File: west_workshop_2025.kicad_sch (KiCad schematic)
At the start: 4 parts

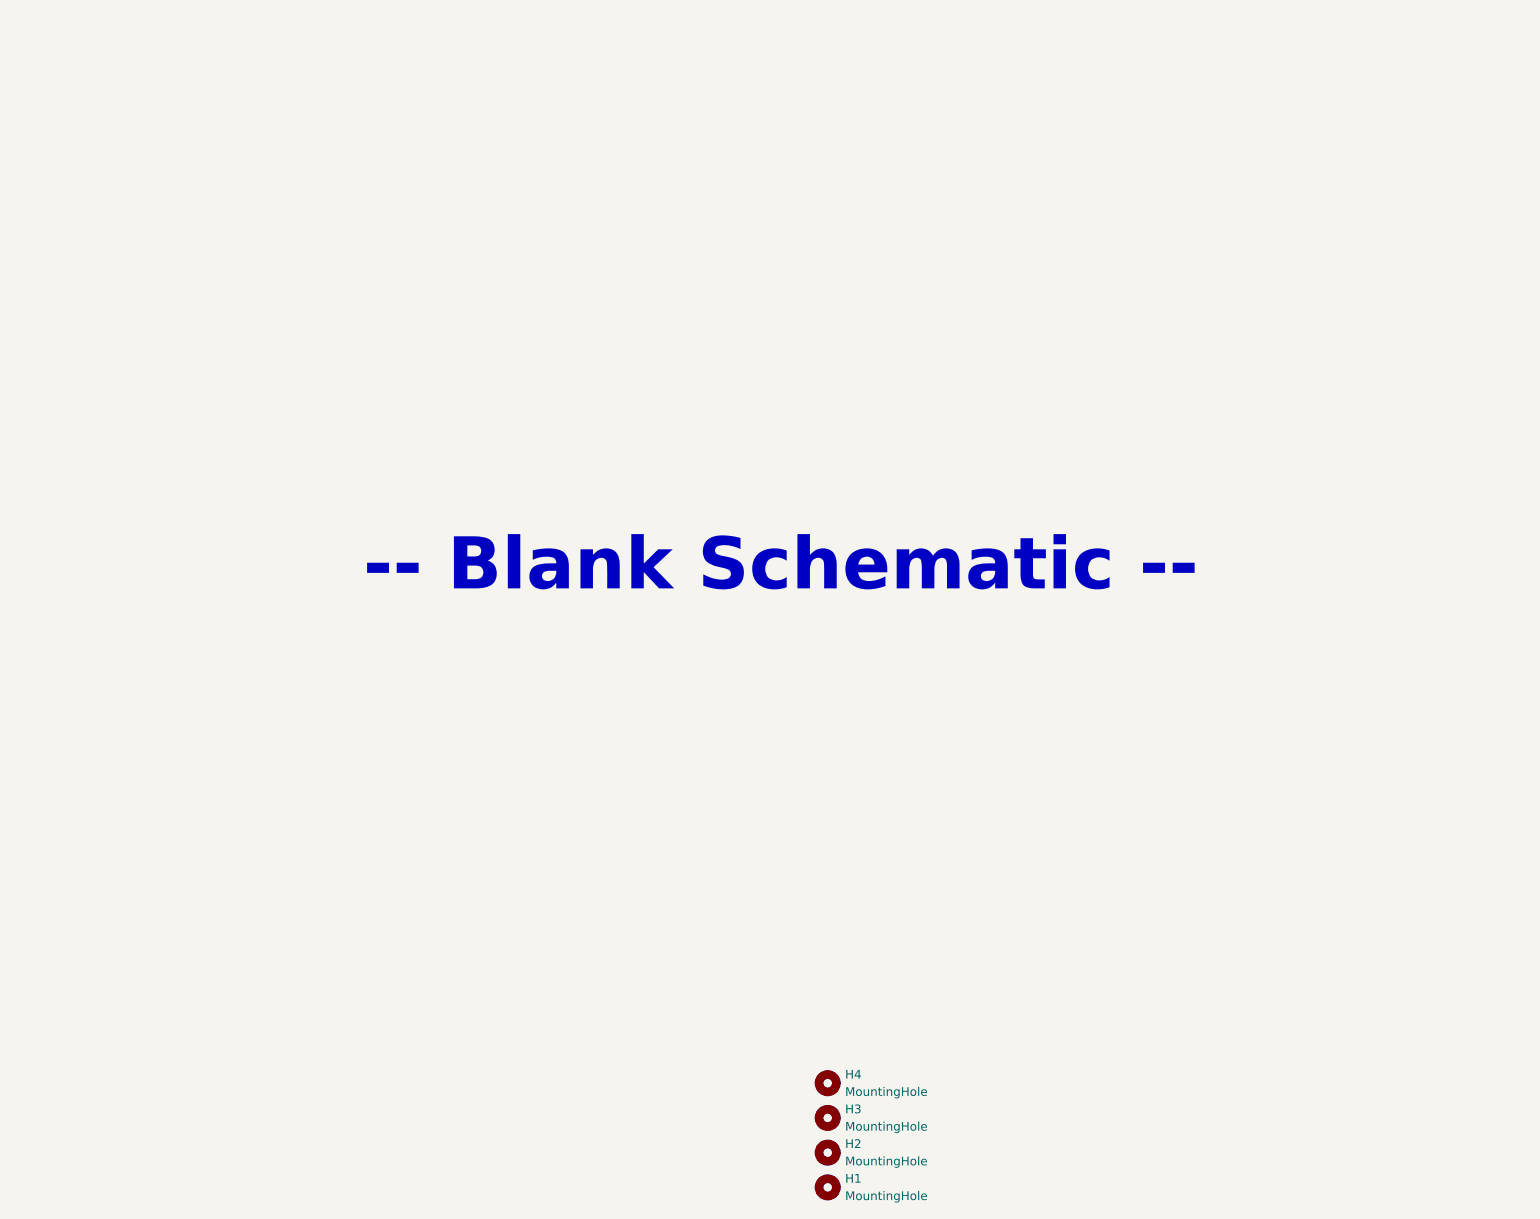
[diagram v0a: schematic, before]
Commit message: Schematic Done - Ready for layout
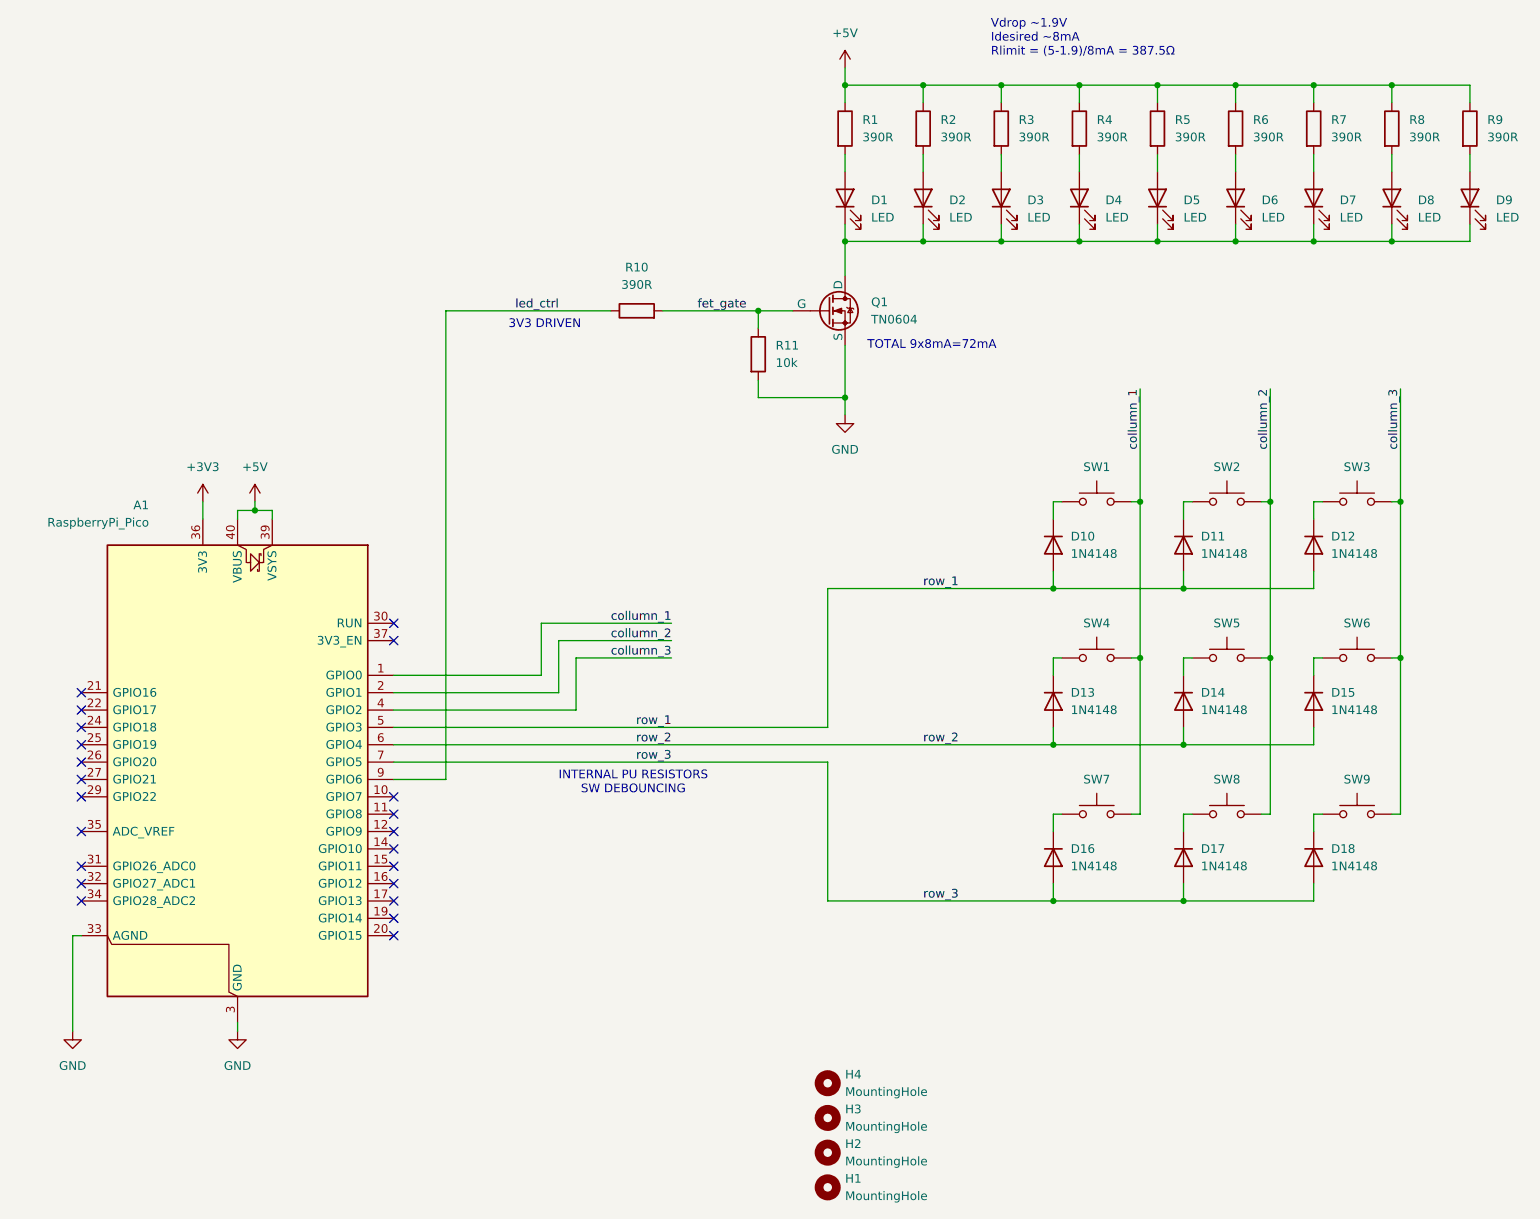
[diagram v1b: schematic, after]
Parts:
- added A1: RaspberryPi_Pico, 0_west_footprints:RaspberryPi_Pico, symbol 0_west_symbols:RaspberryPi_Pico
- added D1, D2, D3, D4, D5, D6, D7, D8, D9: LED, 0_west_footprints:Kingbright_WP914x, symbol 0_west_symbols:LED
- added D10, D11, D12, D13, D14, D15, D16, D17, D18: 1N4148, Diode_THT:D_DO-35_SOD27_P7.62mm_Horizontal, symbol 0_west_symbols:DIODE
- added Q1: TN0604, Package_TO_SOT_THT:TO-92L_Inline, symbol 0_west_symbols:NMOS
- added R1, R10, R2, R3, R4, R5, R6, R7, R8, R9: 390R, Resistor_THT:R_Axial_DIN0204_L3.6mm_D1.6mm_P5.08mm_Horizontal, symbol 0_west_symbols:Resistor
- added R11: 10k, Resistor_THT:R_Axial_DIN0204_L3.6mm_D1.6mm_P5.08mm_Horizontal, symbol 0_west_symbols:Resistor
- added SW1, SW2, SW3, SW4, SW5, SW6, SW7, SW8, SW9: switch_1.00u, 0_west_footprints:SW_Cherry_MX_PCB_1.00u, symbol 0_west_symbols:Switch_Push
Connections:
- new net: D1.1 (K), D2.1 (K), D3.1 (K), D4.1 (K), D5.1 (K), D6.1 (K), D7.1 (K), D8.1 (K), D9.1 (K), Q1.1 (D)
- new net: D1.2 (A), R1.2
- new net: D16.1 (K), SW7.1
- new net: D6.2 (A), R6.2
- new net: D4.2 (A), R4.2
- new net: D17.1 (K), SW8.1
- new net: D15.1 (K), SW6.1
- new net: D9.2 (A), R9.2
- new net: D2.2 (A), R2.2
- new net: D10.1 (K), SW1.1
- new net: D5.2 (A), R5.2
- new net: D14.1 (K), SW5.1
- new net: D13.1 (K), SW4.1
- new net: D3.2 (A), R3.2
- new net: D11.1 (K), SW2.1
- new net: D18.1 (K), SW9.1
- new net: D12.1 (K), SW3.1
- new net: D7.2 (A), R7.2
- new net: D8.2 (A), R8.2
- new net +3V3: A1.36 (3V3)
- new net +5V: A1.39 (VSYS), A1.40 (VBUS), R1.1, R2.1, R3.1, R4.1, R5.1, R6.1, R7.1, R8.1, R9.1
- new net GND: A1.13 (GND), A1.18 (GND), A1.23 (GND), A1.28 (GND), A1.3 (GND), A1.33 (AGND), A1.38 (GND), A1.8 (GND), Q1.3 (S), R11.2
- new net collumn_1: A1.1 (GPIO0), SW1.2, SW4.2, SW7.2
- new net collumn_2: A1.2 (GPIO1), SW2.2, SW5.2, SW8.2
- new net collumn_3: A1.4 (GPIO2), SW3.2, SW6.2, SW9.2
- new net fet_gate: Q1.2 (G), R10.2, R11.1
- new net led_ctrl: A1.9 (GPIO6), R10.1
- new net row_1: A1.5 (GPIO3), D10.2 (A), D11.2 (A), D12.2 (A)
- new net row_2: A1.6 (GPIO4), D13.2 (A), D14.2 (A), D15.2 (A)
- new net row_3: A1.7 (GPIO5), D16.2 (A), D17.2 (A), D18.2 (A)
- no-connect marks 0 -> 22
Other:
- note added: "3V3 DRIVEN"
- note added: "INTERNAL PU RESISTORS SW DEBOUNCING"
- note added: "TOTAL 9x8mA=72mA"
- note added: "Vdrop ~1.9V Idesired ~8mA Rlimit = (5-1.9)/8mA = 387.5Ω"
- note removed: "-- Blank Schematic --"
